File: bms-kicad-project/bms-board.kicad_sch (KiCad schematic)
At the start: 0 parts

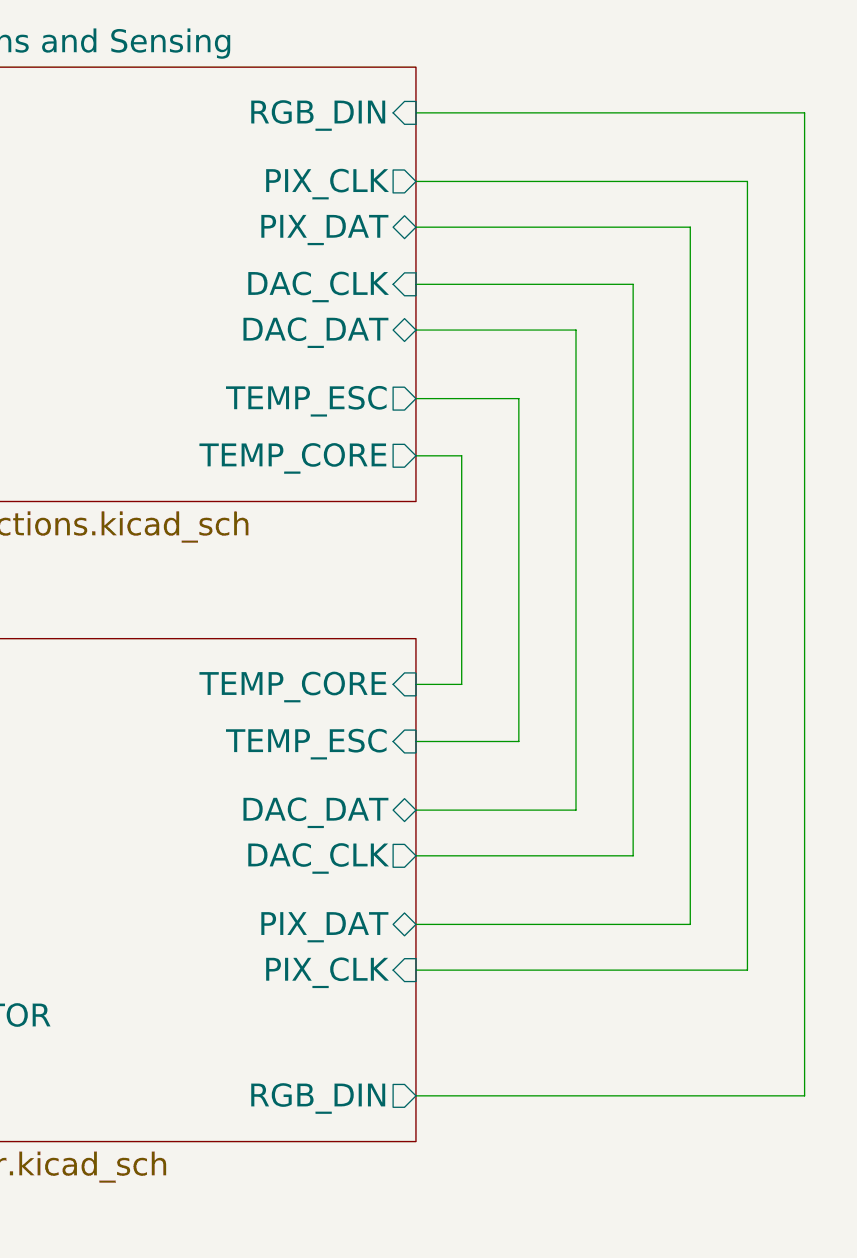
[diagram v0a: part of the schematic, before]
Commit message: feat: biiig layout and slight design change commit
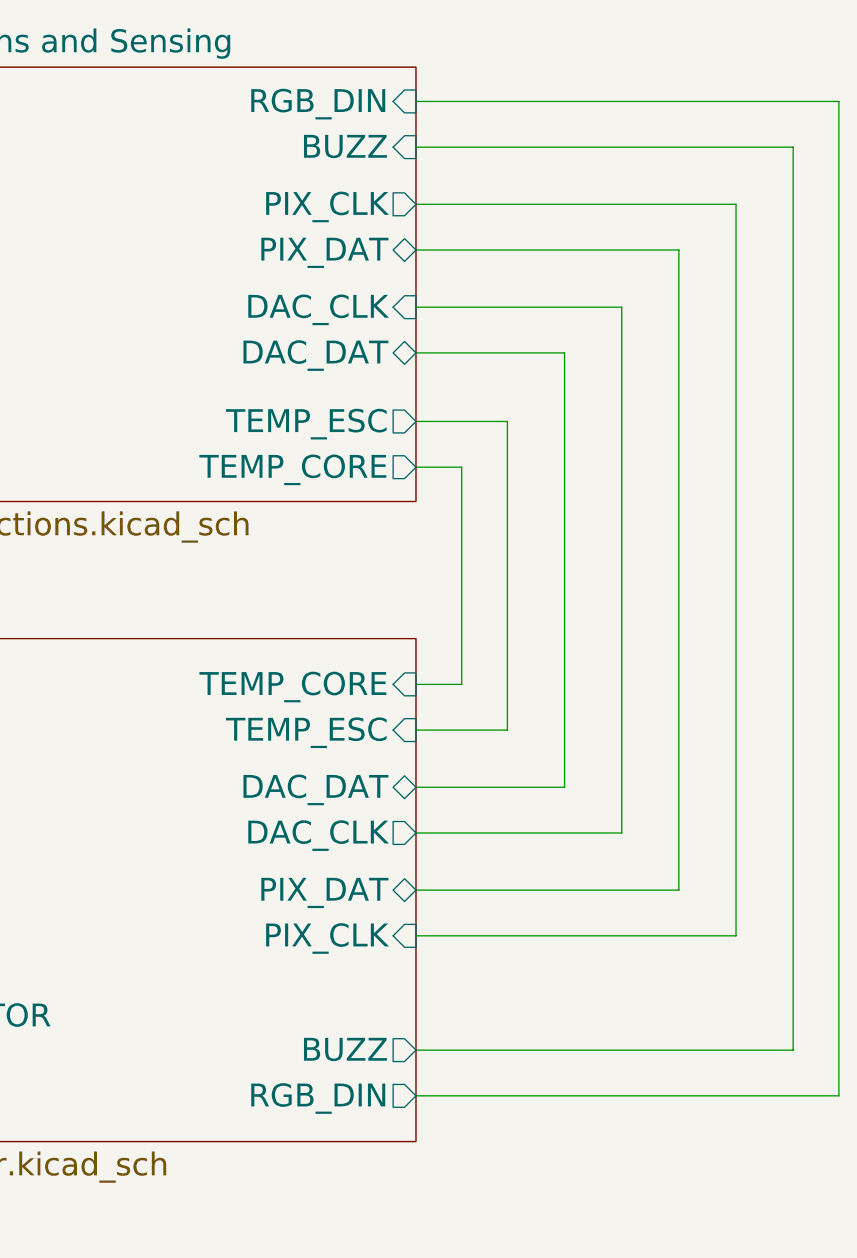
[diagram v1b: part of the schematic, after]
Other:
- sheet External Connections and Sensing ports: added BUZZ; removed none
- sheet Microcontroller ports: added BUZZ; removed none
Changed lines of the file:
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@@
     (company "AeroNU - FixedWing")
   )
-  (wire (pts (xy 359.41 124.46) (xy 359.41 99.06))
+  (wire (pts (xy 359.41 124.46) (xy 359.41 100.33))
     (stroke (width 0) (type default))
   )
@@
     (stroke (width 0) (type default))
   )
-  (wire (pts (xy 354.33 60.96) (xy 397.51 60.96))
-    (stroke (width 0) (type default))
-  )
-  (wire (pts (xy 378.46 80.01) (xy 378.46 143.51))
+  (wire (pts (xy 354.33 59.69) (xy 401.32 59.69))
+    (stroke (width 0) (type default))
+  )
+  (wire (pts (xy 377.19 82.55) (xy 377.19 140.97))
     (stroke (width 0) (type default))
   )
@@
     (stroke (width 0) (type default))
   )
-  (wire (pts (xy 354.33 156.21) (xy 391.16 156.21))
-    (stroke (width 0) (type default))
-  )
-  (wire (pts (xy 397.51 60.96) (xy 397.51 170.18))
-    (stroke (width 0) (type default))
-  )
-  (wire (pts (xy 354.33 130.81) (xy 365.76 130.81))
-    (stroke (width 0) (type default))
-  )
-  (wire (pts (xy 397.51 170.18) (xy 354.33 170.18))
-    (stroke (width 0) (type default))
-  )
-  (wire (pts (xy 365.76 92.71) (xy 365.76 130.81))
-    (stroke (width 0) (type default))
-  )
-  (wire (pts (xy 391.16 68.58) (xy 391.16 156.21))
-    (stroke (width 0) (type default))
-  )
-  (wire (pts (xy 354.33 99.06) (xy 359.41 99.06))
+  (wire (pts (xy 354.33 152.4) (xy 389.89 152.4))
+    (stroke (width 0) (type default))
+  )
+  (wire (pts (xy 401.32 59.69) (xy 401.32 170.18))
+    (stroke (width 0) (type default))
+  )
+  (wire (pts (xy 354.33 129.54) (xy 364.49 129.54))
+    (stroke (width 0) (type default))
+  )
+  (wire (pts (xy 401.32 170.18) (xy 354.33 170.18))
+    (stroke (width 0) (type default))
+  )
+  (wire (pts (xy 364.49 95.25) (xy 364.49 129.54))
+    (stroke (width 0) (type default))
+  )
+  (wire (pts (xy 396.24 64.77) (xy 354.33 64.77))
+    (stroke (width 0) (type default))
+  )
+  (wire (pts (xy 389.89 71.12) (xy 389.89 152.4))
+    (stroke (width 0) (type default))
+  )
+  (wire (pts (xy 354.33 100.33) (xy 359.41 100.33))
     (stroke (width 0) (type default))
   )
@@
     (stroke (width 0) (type default))
   )
-  (wire (pts (xy 384.81 73.66) (xy 384.81 151.13))
+  (wire (pts (xy 383.54 76.2) (xy 383.54 147.32))
     (stroke (width 0) (type default))
   )
@@
     (stroke (width 0) (type default))
   )
-  (wire (pts (xy 354.33 92.71) (xy 365.76 92.71))
-    (stroke (width 0) (type default))
-  )
-  (wire (pts (xy 372.11 138.43) (xy 354.33 138.43))
+  (wire (pts (xy 354.33 95.25) (xy 364.49 95.25))
+    (stroke (width 0) (type default))
+  )
+  (wire (pts (xy 370.84 135.89) (xy 354.33 135.89))
     (stroke (width 0) (type default))
   )
@@
     (stroke (width 0) (type default))
   )
+  (wire (pts (xy 396.24 165.1) (xy 396.24 64.77))
+    (stroke (width 0) (type default))
+  )
   (wire (pts (xy 205.74 156.21) (xy 274.32 156.21))
     (stroke (width 0) (type default))
   )
-  (wire (pts (xy 354.33 80.01) (xy 378.46 80.01))
+  (wire (pts (xy 354.33 82.55) (xy 377.19 82.55))
     (stroke (width 0) (type default))
   )
@@
     (stroke (width 0) (type default))
   )
+  (wire (pts (xy 354.33 165.1) (xy 396.24 165.1))
+    (stroke (width 0) (type default))
+  )
   (wire (pts (xy 205.74 134.62) (xy 274.32 134.62))
     (stroke (width 0) (type default))
@@
     (stroke (width 0) (type default))
   )
-  (wire (pts (xy 354.33 151.13) (xy 384.81 151.13))
-    (stroke (width 0) (type default))
-  )
-  (wire (pts (xy 354.33 68.58) (xy 391.16 68.58))
+  (wire (pts (xy 354.33 147.32) (xy 383.54 147.32))
+    (stroke (width 0) (type default))
+  )
+  (wire (pts (xy 354.33 71.12) (xy 389.89 71.12))
     (stroke (width 0) (type default))
   )
@@
     (stroke (width 0) (type default))
   )
-  (wire (pts (xy 354.33 73.66) (xy 384.81 73.66))
+  (wire (pts (xy 354.33 76.2) (xy 383.54 76.2))
     (stroke (width 0) (type default))
   )
@@
     (stroke (width 0) (type default))
   )
-  (wire (pts (xy 372.11 85.09) (xy 372.11 138.43))
+  (wire (pts (xy 370.84 87.63) (xy 370.84 135.89))
     (stroke (width 0) (type default))
   )
@@
     (stroke (width 0) (type default))
   )
-  (wire (pts (xy 354.33 85.09) (xy 372.11 85.09))
-    (stroke (width 0) (type default))
-  )
-  (wire (pts (xy 354.33 143.51) (xy 378.46 143.51))
+  (wire (pts (xy 354.33 87.63) (xy 370.84 87.63))
+    (stroke (width 0) (type default))
+  )
+  (wire (pts (xy 354.33 140.97) (xy 377.19 140.97))
     (stroke (width 0) (type default))
   )
@@
       (effects (font (size 2.54 2.54)) (justify left))
     )
-    (pin "PIX_DAT" bidirectional (at 354.33 151.13 0)
+    (pin "PIX_DAT" bidirectional (at 354.33 147.32 0)
       (effects (font (size 2.54 2.54)) (justify right))
     )
@@
       (effects (font (size 2.54 2.54)) (justify right))
     )
-    (pin "DAC_DAT" bidirectional (at 354.33 138.43 0)
-      (effects (font (size 2.54 2.54)) (justify right))
-    )
-    (pin "TEMP_ESC" input (at 354.33 130.81 0)
+    (pin "DAC_DAT" bidirectional (at 354.33 135.89 0)
+      (effects (font (size 2.54 2.54)) (justify right))
+    )
+    (pin "TEMP_ESC" input (at 354.33 129.54 0)
       (effects (font (size 2.54 2.54)) (justify right))
     )
@@
       (effects (font (size 2.54 2.54)) (justify left))
     )
-    (pin "DAC_CLK" output (at 354.33 143.51 0)
-      (effects (font (size 2.54 2.54)) (justify right))
-    )
-    (pin "PIX_CLK" input (at 354.33 156.21 0)
+    (pin "DAC_CLK" output (at 354.33 140.97 0)
+      (effects (font (size 2.54 2.54)) (justify right))
+    )
+    (pin "PIX_CLK" input (at 354.33 152.4 0)
       (effects (font (size 2.54 2.54)) (justify right))
     )
     (pin "TEMP_CORE" input (at 354.33 124.46 0)
+      (effects (font (size 2.54 2.54)) (justify right))
+    )
+    (pin "BUZZ" output (at 354.33 165.1 0)
       (effects (font (size 2.54 2.54)) (justify right))
     )
@@
       (effects (font (size 2.54 2.54)) (justify left top))
     )
-    (pin "PIX_DAT" bidirectional (at 354.33 73.66 0)
+    (pin "PIX_DAT" bidirectional (at 354.33 76.2 0)
       (effects (font (size 2.54 2.54)) (justify right))
     )
@@
       (effects (font (size 2.54 2.54)) (justify left))
     )
-    (pin "RGB_DIN" input (at 354.33 60.96 0)
-      (effects (font (size 2.54 2.54)) (justify right))
-    )
-    (pin "DAC_DAT" bidirectional (at 354.33 85.09 0)
-      (effects (font (size 2.54 2.54)) (justify right))
-    )
-    (pin "DAC_CLK" input (at 354.33 80.01 0)
-      (effects (font (size 2.54 2.54)) (justify right))
-    )
-    (pin "PIX_CLK" output (at 354.33 68.58 0)
-      (effects (font (size 2.54 2.54)) (justify right))
-    )
-    (pin "TEMP_CORE" output (at 354.33 99.06 0)
-      (effects (font (size 2.54 2.54)) (justify right))
-    )
-    (pin "TEMP_ESC" output (at 354.33 92.71 0)
-      (effects (font (size 2.54 2.54)) (justify right))
-    )
+    (pin "RGB_DIN" input (at 354.33 59.69 0)
+      (effects (font (size 2.54 2.54)) (justify right))
+    )
+    (pin "DAC_DAT" bidirectional (at 354.33 87.63 0)
+      (effects (font (size 2.54 2.54)) (justify right))
+    )
+    (pin "DAC_CLK" input (at 354.33 82.55 0)
+      (effects (font (size 2.54 2.54)) (justify right))
+    )
+    (pin "PIX_CLK" output (at 354.33 71.12 0)
+      (effects (font (size 2.54 2.54)) (justify right))
+    )
+    (pin "TEMP_CORE" output (at 354.33 100.33 0)
+      (effects (font (size 2.54 2.54)) (justify right))
+    )
+    (pin "TEMP_ESC" output (at 354.33 95.25 0)
+      (effects (font (size 2.54 2.54)) (justify right))
+    )
+    (pin "BUZZ" input (at 354.33 64.77 0)
+      (effects (font (size 2.54 2.54)) (justify right))
+    )

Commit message: feat:bos->lax layout sesh
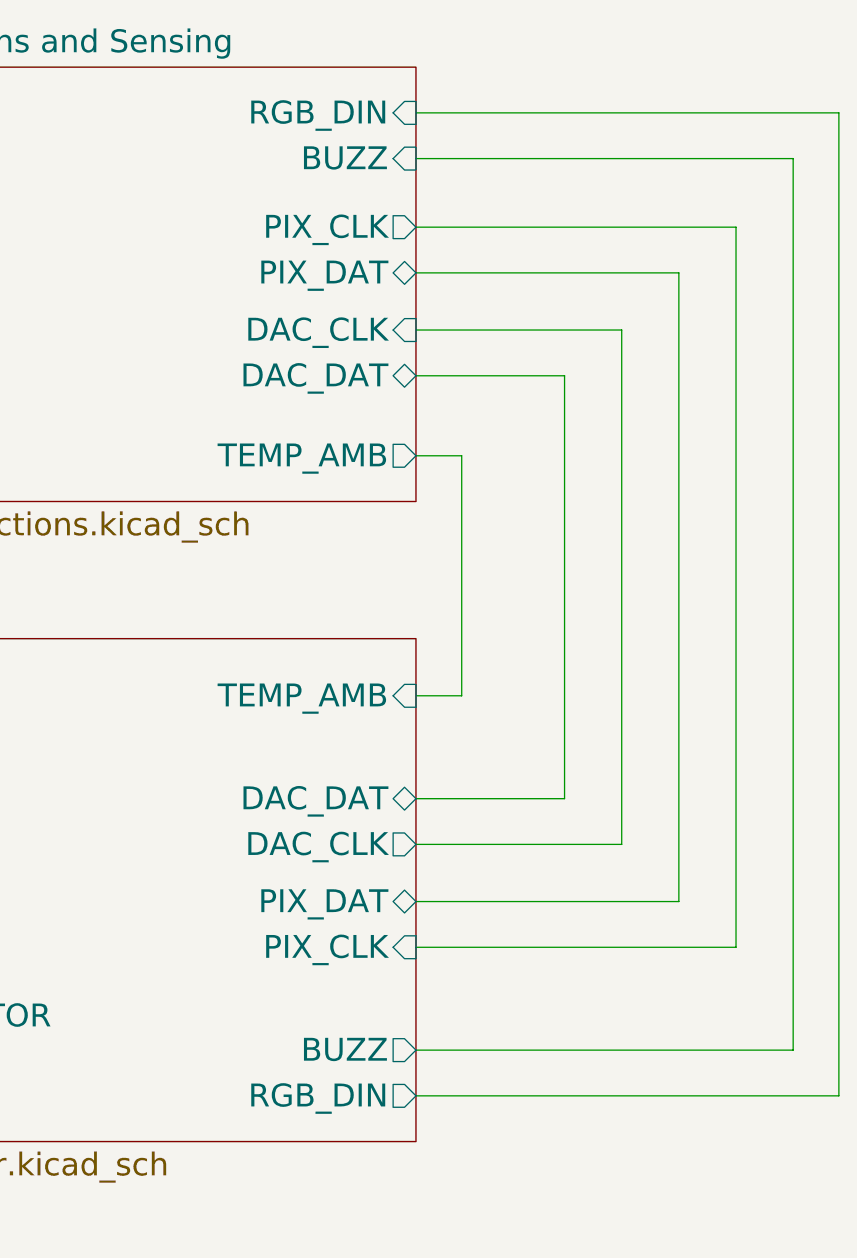
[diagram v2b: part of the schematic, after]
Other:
- sheet External Connections and Sensing ports: added TEMP_AMB; removed TEMP_CORE, TEMP_ESC
- sheet Microcontroller ports: added TEMP_AMB; removed TEMP_CORE, TEMP_ESC
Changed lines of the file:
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@@
     (company "AeroNU - FixedWing")
   )
-  (wire (pts (xy 359.41 124.46) (xy 359.41 100.33))
+  (wire (pts (xy 359.41 125.73) (xy 359.41 99.06))
     (stroke (width 0) (type default))
   )
@@
     (stroke (width 0) (type default))
   )
-  (wire (pts (xy 354.33 59.69) (xy 401.32 59.69))
-    (stroke (width 0) (type default))
-  )
-  (wire (pts (xy 377.19 82.55) (xy 377.19 140.97))
+  (wire (pts (xy 354.33 60.96) (xy 401.32 60.96))
+    (stroke (width 0) (type default))
+  )
+  (wire (pts (xy 377.19 85.09) (xy 377.19 142.24))
     (stroke (width 0) (type default))
   )
@@
     (stroke (width 0) (type default))
   )
-  (wire (pts (xy 354.33 152.4) (xy 389.89 152.4))
-    (stroke (width 0) (type default))
-  )
-  (wire (pts (xy 401.32 59.69) (xy 401.32 170.18))
-    (stroke (width 0) (type default))
-  )
-  (wire (pts (xy 354.33 129.54) (xy 364.49 129.54))
+  (wire (pts (xy 354.33 153.67) (xy 389.89 153.67))
+    (stroke (width 0) (type default))
+  )
+  (wire (pts (xy 401.32 60.96) (xy 401.32 170.18))
     (stroke (width 0) (type default))
   )
@@
     (stroke (width 0) (type default))
   )
-  (wire (pts (xy 364.49 95.25) (xy 364.49 129.54))
-    (stroke (width 0) (type default))
-  )
-  (wire (pts (xy 396.24 64.77) (xy 354.33 64.77))
-    (stroke (width 0) (type default))
-  )
-  (wire (pts (xy 389.89 71.12) (xy 389.89 152.4))
-    (stroke (width 0) (type default))
-  )
-  (wire (pts (xy 354.33 100.33) (xy 359.41 100.33))
+  (wire (pts (xy 396.24 66.04) (xy 354.33 66.04))
+    (stroke (width 0) (type default))
+  )
+  (wire (pts (xy 389.89 73.66) (xy 389.89 153.67))
+    (stroke (width 0) (type default))
+  )
+  (wire (pts (xy 354.33 99.06) (xy 359.41 99.06))
     (stroke (width 0) (type default))
   )
@@
     (stroke (width 0) (type default))
   )
-  (wire (pts (xy 383.54 76.2) (xy 383.54 147.32))
+  (wire (pts (xy 383.54 78.74) (xy 383.54 148.59))
     (stroke (width 0) (type default))
   )
@@
     (stroke (width 0) (type default))
   )
-  (wire (pts (xy 354.33 95.25) (xy 364.49 95.25))
-    (stroke (width 0) (type default))
-  )
-  (wire (pts (xy 370.84 135.89) (xy 354.33 135.89))
+  (wire (pts (xy 370.84 137.16) (xy 354.33 137.16))
     (stroke (width 0) (type default))
   )
@@
     (stroke (width 0) (type default))
   )
-  (wire (pts (xy 396.24 165.1) (xy 396.24 64.77))
+  (wire (pts (xy 396.24 165.1) (xy 396.24 66.04))
     (stroke (width 0) (type default))
   )
@@
     (stroke (width 0) (type default))
   )
-  (wire (pts (xy 354.33 82.55) (xy 377.19 82.55))
+  (wire (pts (xy 354.33 85.09) (xy 377.19 85.09))
     (stroke (width 0) (type default))
   )
@@
     (stroke (width 0) (type default))
   )
-  (wire (pts (xy 354.33 147.32) (xy 383.54 147.32))
-    (stroke (width 0) (type default))
-  )
-  (wire (pts (xy 354.33 71.12) (xy 389.89 71.12))
-    (stroke (width 0) (type default))
-  )
-  (wire (pts (xy 354.33 124.46) (xy 359.41 124.46))
-    (stroke (width 0) (type default))
-  )
-  (wire (pts (xy 354.33 76.2) (xy 383.54 76.2))
+  (wire (pts (xy 354.33 148.59) (xy 383.54 148.59))
+    (stroke (width 0) (type default))
+  )
+  (wire (pts (xy 354.33 73.66) (xy 389.89 73.66))
+    (stroke (width 0) (type default))
+  )
+  (wire (pts (xy 354.33 125.73) (xy 359.41 125.73))
+    (stroke (width 0) (type default))
+  )
+  (wire (pts (xy 354.33 78.74) (xy 383.54 78.74))
     (stroke (width 0) (type default))
   )
@@
     (stroke (width 0) (type default))
   )
-  (wire (pts (xy 370.84 87.63) (xy 370.84 135.89))
+  (wire (pts (xy 370.84 90.17) (xy 370.84 137.16))
     (stroke (width 0) (type default))
   )
@@
     (stroke (width 0) (type default))
   )
-  (wire (pts (xy 354.33 87.63) (xy 370.84 87.63))
-    (stroke (width 0) (type default))
-  )
-  (wire (pts (xy 354.33 140.97) (xy 377.19 140.97))
+  (wire (pts (xy 354.33 90.17) (xy 370.84 90.17))
+    (stroke (width 0) (type default))
+  )
+  (wire (pts (xy 354.33 142.24) (xy 377.19 142.24))
     (stroke (width 0) (type default))
   )
@@
       (effects (font (size 2.54 2.54)) (justify left))
     )
-    (pin "PIX_DAT" bidirectional (at 354.33 147.32 0)
+    (pin "PIX_DAT" bidirectional (at 354.33 148.59 0)
       (effects (font (size 2.54 2.54)) (justify right))
     )
@@
       (effects (font (size 2.54 2.54)) (justify right))
     )
-    (pin "DAC_DAT" bidirectional (at 354.33 135.89 0)
-      (effects (font (size 2.54 2.54)) (justify right))
-    )
-    (pin "TEMP_ESC" input (at 354.33 129.54 0)
+    (pin "DAC_DAT" bidirectional (at 354.33 137.16 0)
       (effects (font (size 2.54 2.54)) (justify right))
     )
@@
       (effects (font (size 2.54 2.54)) (justify left))
     )
-    (pin "DAC_CLK" output (at 354.33 140.97 0)
-      (effects (font (size 2.54 2.54)) (justify right))
-    )
-    (pin "PIX_CLK" input (at 354.33 152.4 0)
-      (effects (font (size 2.54 2.54)) (justify right))
-    )
-    (pin "TEMP_CORE" input (at 354.33 124.46 0)
+    (pin "DAC_CLK" output (at 354.33 142.24 0)
+      (effects (font (size 2.54 2.54)) (justify right))
+    )
+    (pin "PIX_CLK" input (at 354.33 153.67 0)
+      (effects (font (size 2.54 2.54)) (justify right))
+    )
+    (pin "TEMP_AMB" input (at 354.33 125.73 0)
       (effects (font (size 2.54 2.54)) (justify right))
     )
@@
       (effects (font (size 2.54 2.54)) (justify left top))
     )
-    (pin "PIX_DAT" bidirectional (at 354.33 76.2 0)
+    (pin "PIX_DAT" bidirectional (at 354.33 78.74 0)
       (effects (font (size 2.54 2.54)) (justify right))
     )
@@
       (effects (font (size 2.54 2.54)) (justify left))
     )
-    (pin "RGB_DIN" input (at 354.33 59.69 0)
-      (effects (font (size 2.54 2.54)) (justify right))
-    )
-    (pin "DAC_DAT" bidirectional (at 354.33 87.63 0)
-      (effects (font (size 2.54 2.54)) (justify right))
-    )
-    (pin "DAC_CLK" input (at 354.33 82.55 0)
-      (effects (font (size 2.54 2.54)) (justify right))
-    )
-    (pin "PIX_CLK" output (at 354.33 71.12 0)
-      (effects (font (size 2.54 2.54)) (justify right))
-    )
-    (pin "TEMP_CORE" output (at 354.33 100.33 0)
-      (effects (font (size 2.54 2.54)) (justify right))
-    )
-    (pin "TEMP_ESC" output (at 354.33 95.25 0)
-      (effects (font (size 2.54 2.54)) (justify right))
-    )
-    (pin "BUZZ" input (at 354.33 64.77 0)
-      (effects (font (size 2.54 2.54)) (justify right))
-    )
+    (pin "RGB_DIN" input (at 354.33 60.96 0)
+      (effects (font (size 2.54 2.54)) (justify right))
+    )
+    (pin "DAC_DAT" bidirectional (at 354.33 90.17 0)
+      (effects (font (size 2.54 2.54)) (justify right))
+    )
+    (pin "DAC_CLK" input (at 354.33 85.09 0)
+      (effects (font (size 2.54 2.54)) (justify right))
+    )
+    (pin "PIX_CLK" output (at 354.33 73.66 0)
+      (effects (font (size 2.54 2.54)) (justify right))
+    )
+    (pin "TEMP_AMB" output (at 354.33 99.06 0)
+      (effects (font (size 2.54 2.54)) (justify right))
+    )
+    (pin "BUZZ" input (at 354.33 66.04 0)
+      (effects (font (size 2.54 2.54)) (justify right))
+    )
